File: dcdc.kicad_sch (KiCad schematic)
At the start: 35 parts, among them J10 Conn_01x01, J11 Conn_01x01, J12 Conn_01x01, J8 Conn_01x01, J9 Conn_01x01, T1 Transformer_SP_1S, U1 L78L33_SOT89, U2 TMP117, U3 LT3439

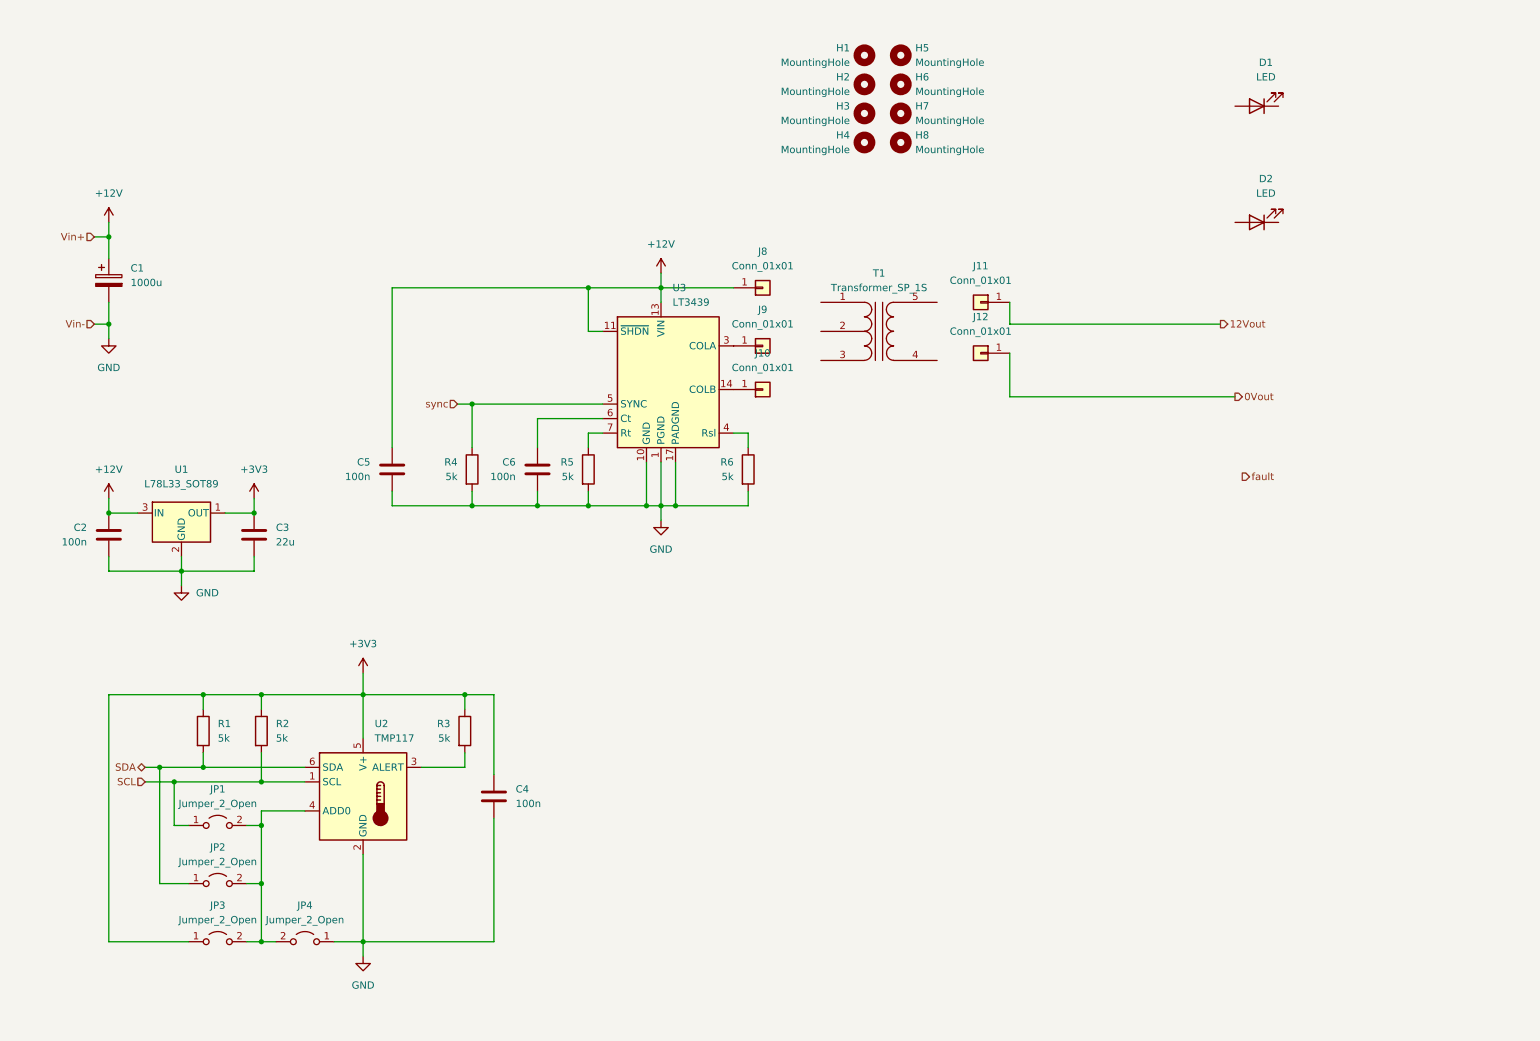
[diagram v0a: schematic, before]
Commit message: asdf
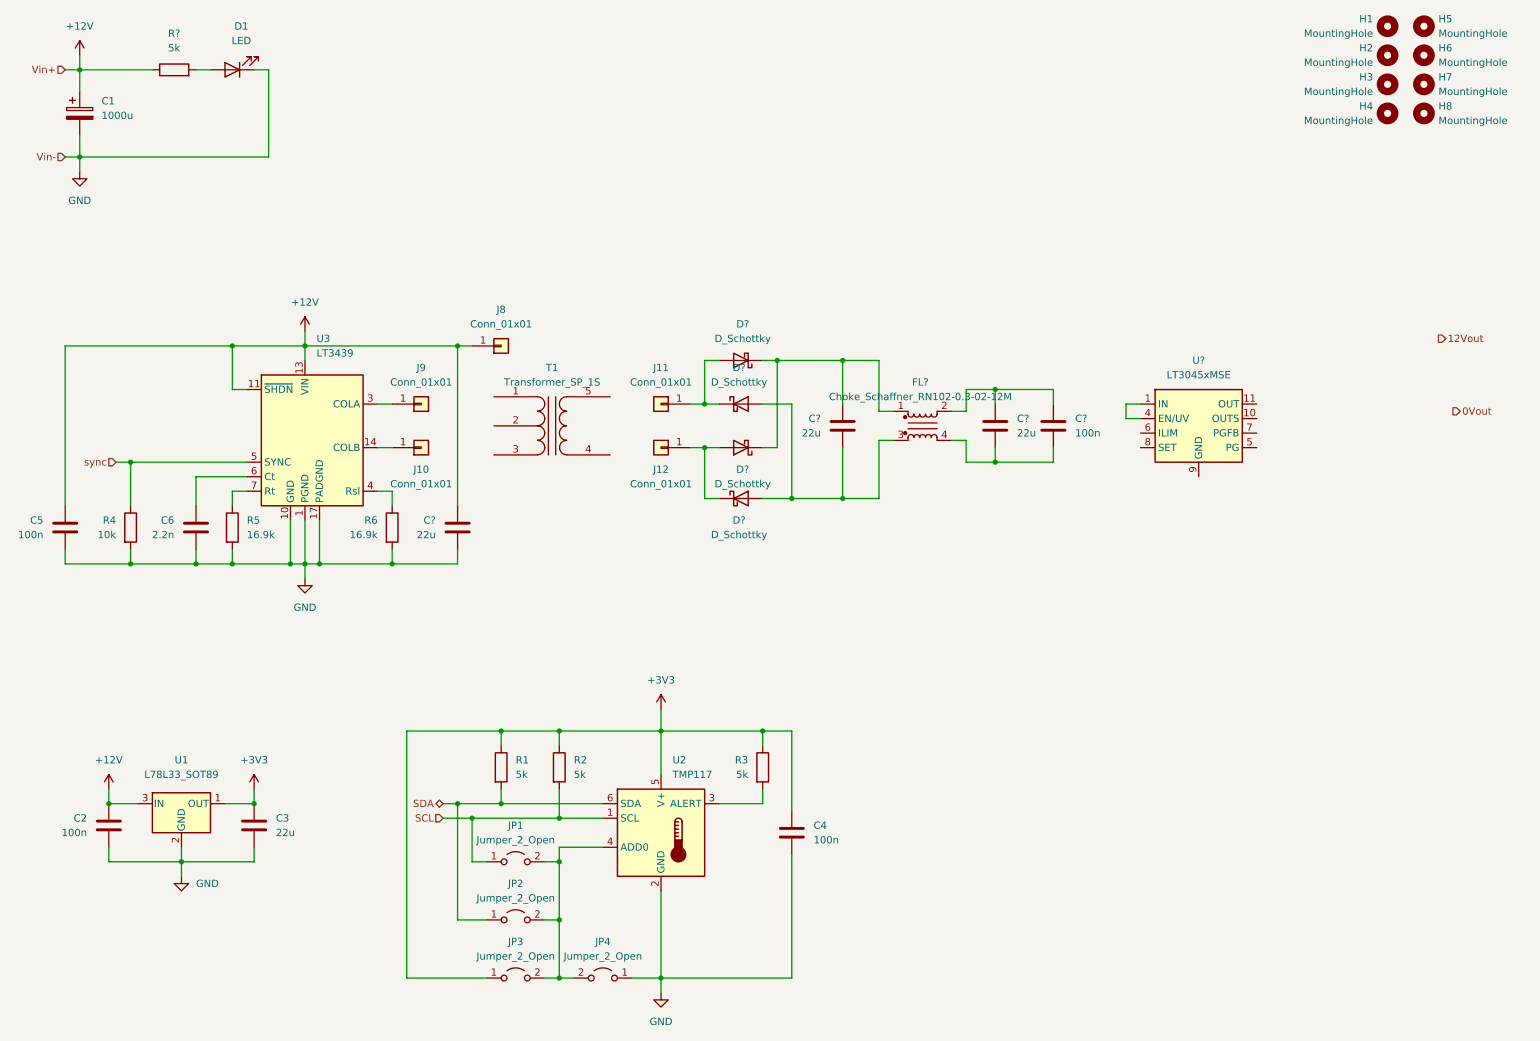
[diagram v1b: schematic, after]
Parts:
- removed D2: LED, LED_SMD:LED_1206_3216Metric, symbol Device:LED
- added C? (x3): 22u, Capacitor_SMD:C_1206_3216Metric, symbol Device:C
- added C?: 100n, Capacitor_SMD:C_0805_2012Metric, symbol Device:C
- added D? (x4): D_Schottky, Diode_SMD:D_SOD-123F, symbol Device:D_Schottky
- added FL?: Choke_Schaffner_RN102-0.3-02-12M, Inductor_THT:Choke_Schaffner_RN102-04-14.0x14.0mm, symbol Filter:Choke_Schaffner_RN102-0.3-02-12M
- added R?: 5k, Resistor_SMD:R_0805_2012Metric, symbol Device:R
- added U?: LT3045xMSE, Package_SO:MSOP-12-1EP_3x4mm_P0.65mm_EP1.65x2.85mm, symbol Regulator_Linear:LT3045xMSE
- C3: footprint Capacitor_SMD:C_0805_2012Metric -> Capacitor_SMD:C_1206_3216Metric
- C6: value 100n -> 2.2n
- R4: value 5k -> 10k
- R5, R6: value 5k -> 16.9k
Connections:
- net +12V: now also C?.1, R?.1
- net 0Vout: no longer J12.1 (Pin_1)
- net 12Vout: no longer J11.1 (Pin_1)
- net GND: now also D1.1 (K), C?.2
- net at D1.2 (A): now also R?.2
- new net: C?.1, D?.1 (K), D?.1 (K), FL?.1
- new net: D?.1 (K), D?.2 (A), J11.1 (Pin_1)
- new net: C?.2, D?.2 (A), D?.2 (A), FL?.3
- new net: C?.1, C?.1, FL?.2
- new net: C?.2, C?.2, FL?.4
- new net: D?.1 (K), D?.2 (A), J12.1 (Pin_1)
- new net: U?.1 (IN), U?.2 (IN), U?.3 (IN), U?.4 (EN/UV)
- new net: U?.11 (OUT), U?.12 (OUT)
- new net: U?.13 (GND), U?.9 (GND)
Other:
- moved on the sheet: C1, C2, C3, C4, C5, C6, D1, H1, H2, H3, H4, H5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
